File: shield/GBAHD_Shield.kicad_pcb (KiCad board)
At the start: 2 copper layers, 53.4 x 53.1 mm, 38 parts, among them J1 Conn_01x01, J10 Conn_01x10, J11 Conn_02x03_Odd_Even, J12 Conn_01x01, J2 FFC_OGBA_32, J3 FFC_GBA-SP, J4 Conn_01x16, J5 FFC_OGBA_40, J6 Conn_01x06, J7 Conn_01x08, J8 Conn_01x10, J9 Conn_01x08, Q1 Q_PMOS_GSD, SW1 SW_Push, T1 Conn_01x01, T2 Conn_01x01, T3 Conn_01x01, T4 Conn_01x01, T5 Conn_01x01, T6 Conn_01x01, T7 Conn_01x01, T8 Conn_01x01, U1 AMS1117-ADJ, U2 74HC595, U3 74HC595, U4 SNES_7PIN, U5 ATmega328P-AU

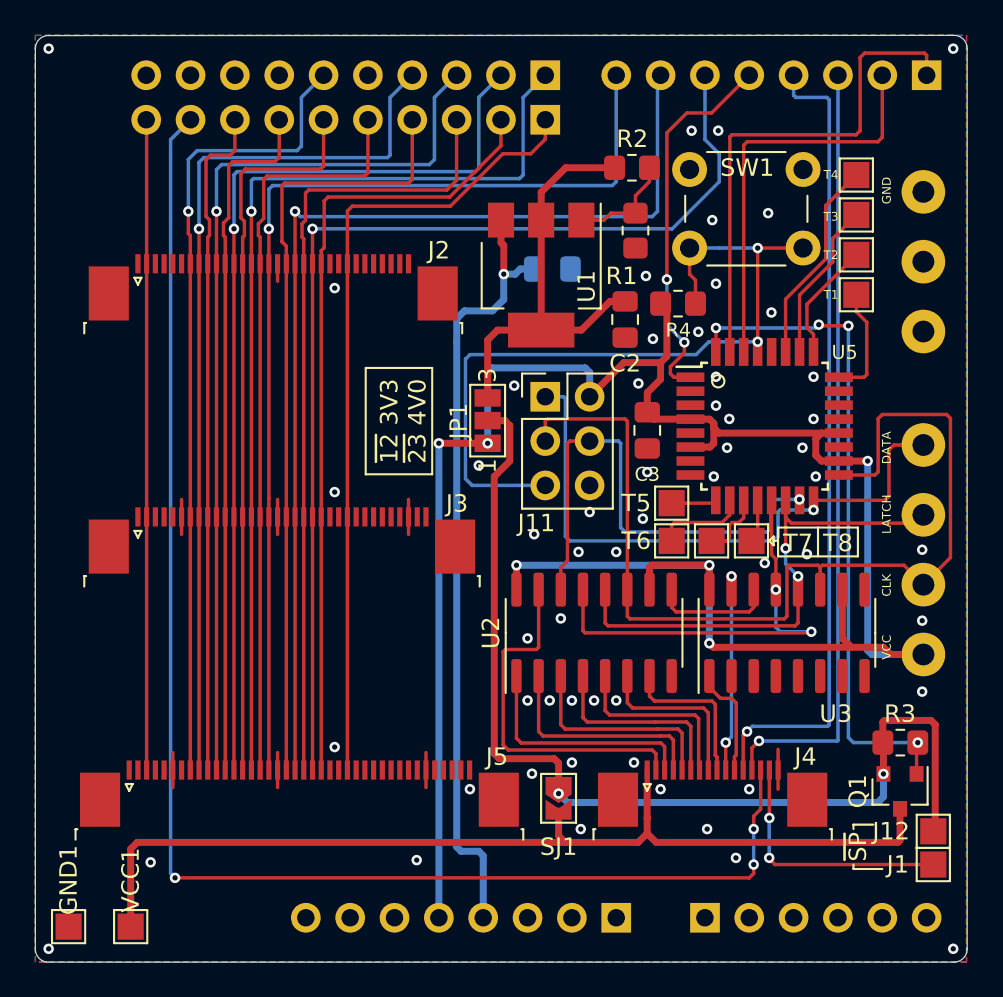
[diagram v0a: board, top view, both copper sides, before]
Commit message: Cleanup for shield pcb
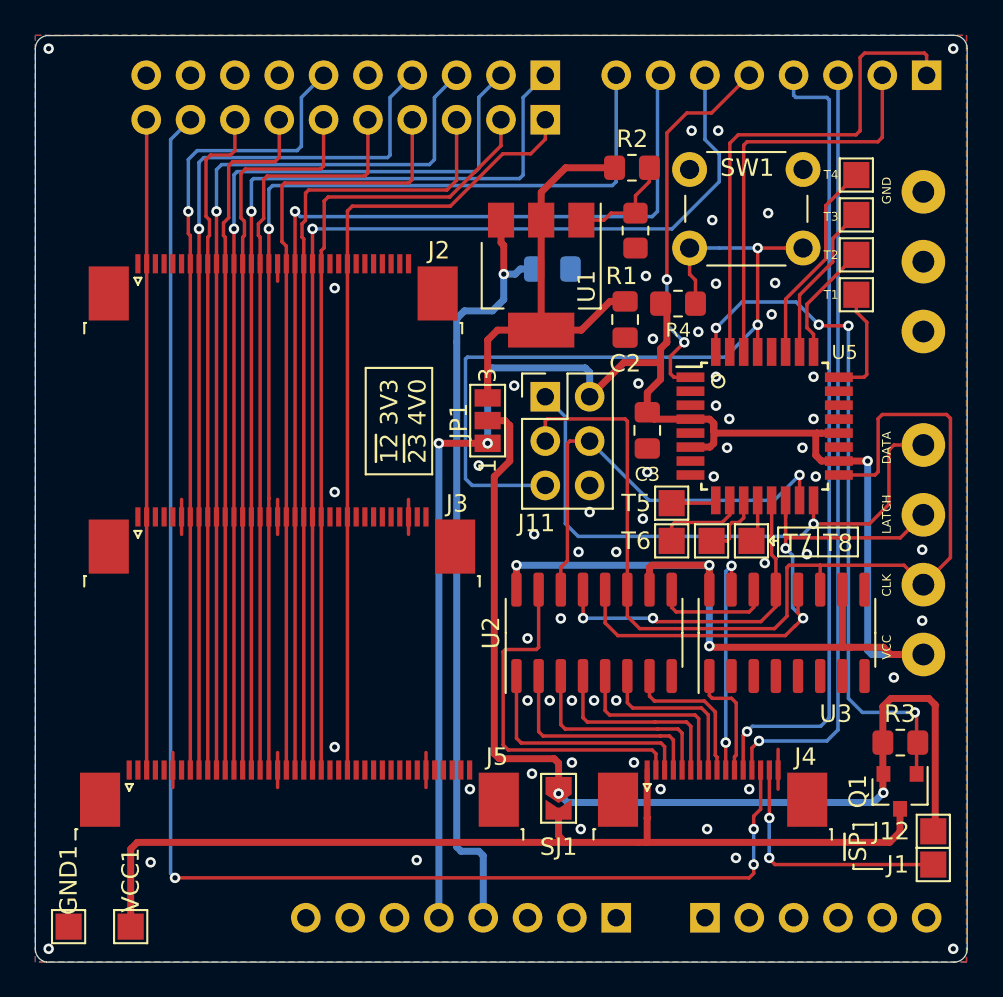
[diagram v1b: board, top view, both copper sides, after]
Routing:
- net ~GBA_BUTTONS_EN~: track 25.0 -> 19.3 mm
- net SNS_LATCH: track 29.7 -> 33.1 mm
- net ICSP_MOSI: track 28.6 -> 25.3 mm
- net VCC: track 57.9 -> 60.0 mm
- net GBA_START: track 11.2 -> 13.2 mm
- net GBA_POWER_SEL: track 38.6 -> 39.2 mm
- net GND: vias 57 -> 58
